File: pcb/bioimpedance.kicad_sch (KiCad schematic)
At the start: 44 parts, among them J1 Conn_01x05_Pin, J3 USB_C_Receptacle_USB2.0_16P, J6 Conn_01x16_Pin, J8 Conn_01x16_Pin, SW5 SW_Push, SW6 SW_Push, U1 ESP32-S3-WROOM-1, U2 MAX30001CWV_T, U3 AP2112K-3.3, U4 AP2112K-1.8, Y1 OK322532.768KJBA4SL

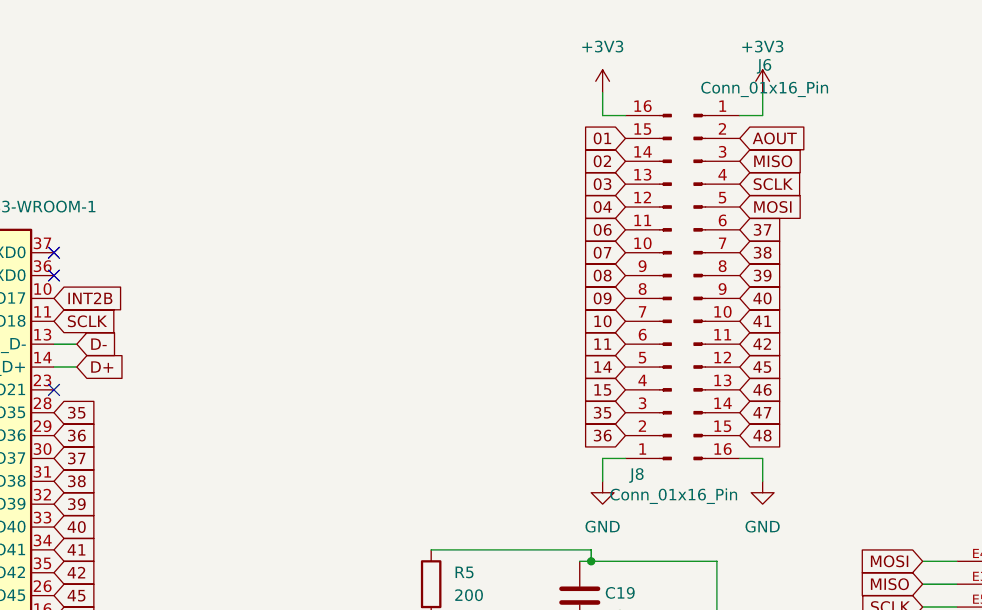
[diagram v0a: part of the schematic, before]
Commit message: reroute pcb
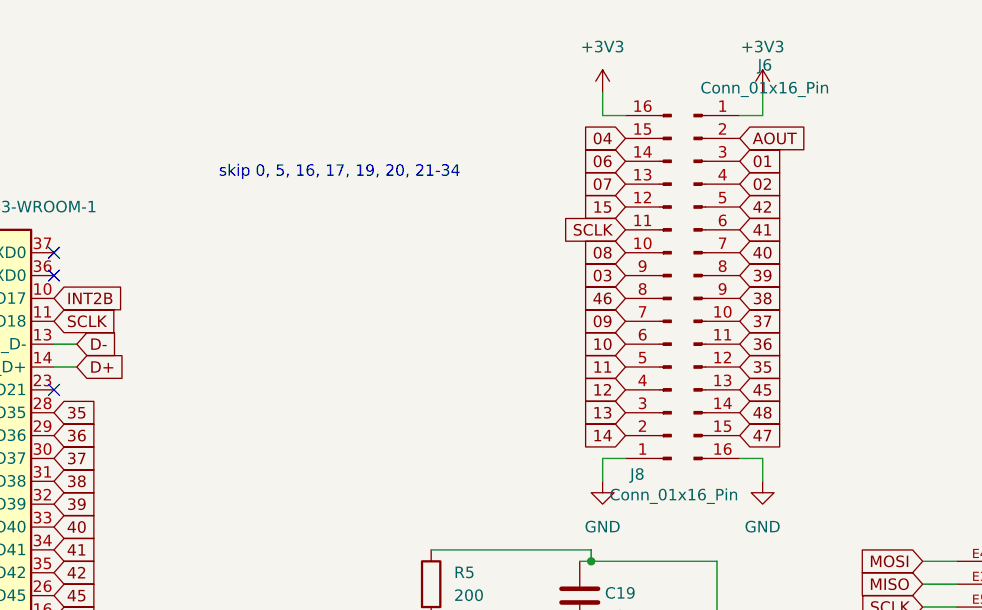
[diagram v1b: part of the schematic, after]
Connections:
- net 01: now also J6.3 (Pin_3); no longer J8.15 (Pin_15)
- net 02: now also J6.4 (Pin_4); no longer J8.14 (Pin_14)
- net 03: now also J8.9 (Pin_9); no longer J8.13 (Pin_13)
- net 04: now also J8.15 (Pin_15); no longer J8.12 (Pin_12)
- net 06: now also J8.14 (Pin_14); no longer J8.11 (Pin_11)
- net 07: now also J8.13 (Pin_13); no longer J8.10 (Pin_10)
- net 08: now also J8.10 (Pin_10); no longer J8.9 (Pin_9)
- net 09: now also J8.7 (Pin_7); no longer J8.8 (Pin_8)
- net 10: now also J8.6 (Pin_6); no longer J8.7 (Pin_7)
- net 11: now also J8.5 (Pin_5); no longer J8.6 (Pin_6)
- net 14: now also J8.2 (Pin_2); no longer J8.5 (Pin_5)
- net 15: now also J8.12 (Pin_12); no longer J8.4 (Pin_4)
- net 35: now also J6.12 (Pin_12); no longer J8.3 (Pin_3)
- net 36: now also J6.11 (Pin_11); no longer J8.2 (Pin_2)
- net 37: now also J6.10 (Pin_10); no longer J6.6 (Pin_6)
- net 38: now also J6.9 (Pin_9); no longer J6.7 (Pin_7)
- net 40: now also J6.7 (Pin_7); no longer J6.9 (Pin_9)
- net 41: now also J6.6 (Pin_6); no longer J6.10 (Pin_10)
- net 42: now also J6.5 (Pin_5); no longer J6.11 (Pin_11)
- net 45: now also J6.13 (Pin_13); no longer J6.12 (Pin_12)
- net 46: now also J8.8 (Pin_8); no longer J6.13 (Pin_13)
- net 47: now also J6.15 (Pin_15); no longer J6.14 (Pin_14)
- net 48: now also J6.14 (Pin_14); no longer J6.15 (Pin_15)
- net MISO: no longer J6.3 (Pin_3)
- net MOSI: no longer J6.5 (Pin_5)
- net SCLK: now also J8.11 (Pin_11); no longer J6.4 (Pin_4)
- new net 12: J8.4 (Pin_4)
- new net 13: J8.3 (Pin_3)
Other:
- note added: "skip 0, 5, 16, 17, 19, 20, 21-34"

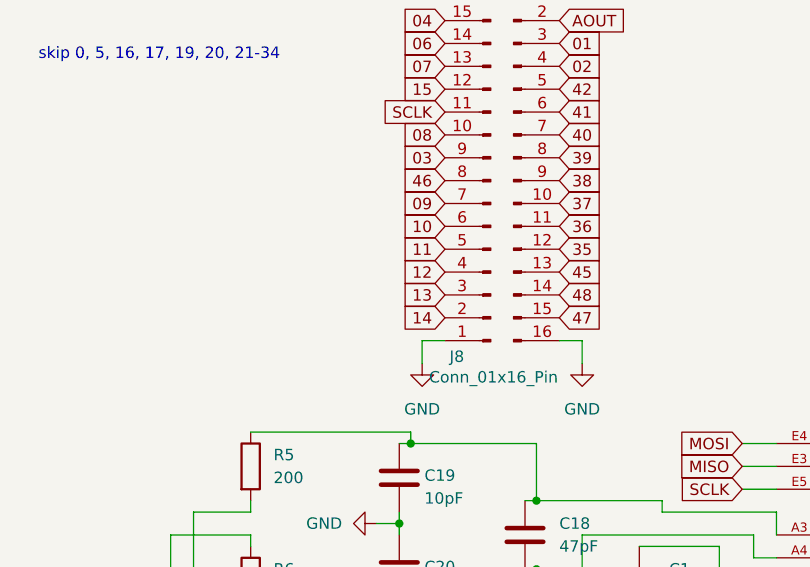
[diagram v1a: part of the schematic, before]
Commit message: reroute pcb
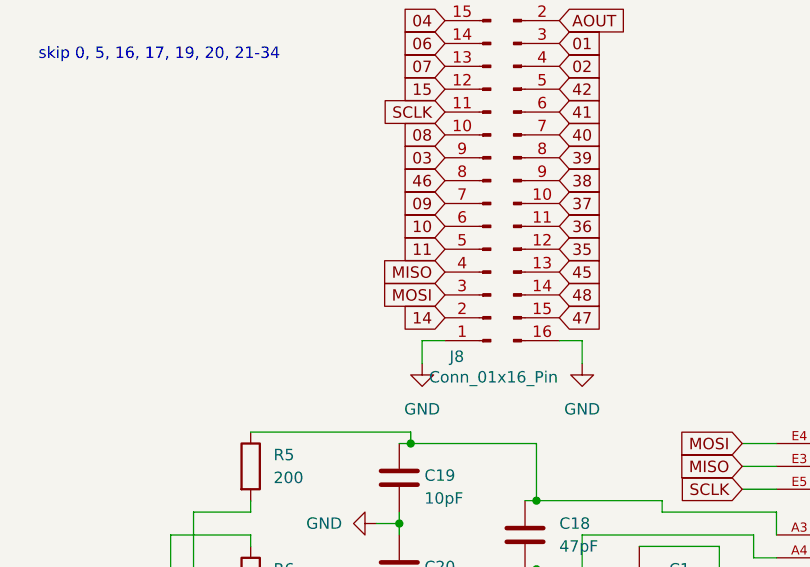
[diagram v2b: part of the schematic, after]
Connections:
- net 12 is gone; now on net MISO: J8.4 (Pin_4)
- net 13 is gone; now on net MOSI: J8.3 (Pin_3)
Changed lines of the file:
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@@
 		)
 	)
-	(global_label "13"
+	(global_label "MOSI"
 		(shape input)
 		(at 158.75 62.23 180)
@@
 		)
 		(property "Intersheetrefs" "${INTERSHEET_REFS}"
-			(at 153.3458 62.23 0)
+			(at 151.1686 62.23 0)
 			(effects
 				(font
@@
 		)
 	)
-	(global_label "12"
+	(global_label "MISO"
 		(shape input)
 		(at 158.75 59.69 180)
@@
 		)
 		(property "Intersheetrefs" "${INTERSHEET_REFS}"
-			(at 153.3458 59.69 0)
-			(effects
-				(font
+			(at 151.1686 59.69 0)
+			(effects
+				(font
